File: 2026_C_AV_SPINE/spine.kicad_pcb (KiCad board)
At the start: 4 copper layers, 165 x 80 mm, 165 parts, among them IC1 LT3960EMSE#TRPBF, J1 Conn_01x02_Socket, J10 Conn_01x02_Socket, J11 DIN41612_02x16_AB, J12 SS-12800-009, J13 SS-12800-009, J14 Conn_01x02_Socket, J2 DIN41612_02x16_AB, J3 Conn_01x02_Socket, J4 SS-12800-009, J5 DIN41612_02x16_AB, J6 DIN41612_02x16_AB, J7 Conn_01x02_Socket, J8 SS-12800-009, J9 Conn_01x02_Socket, Q1 PMOS, Q10 SI7972DP-T1-GE3, Q11 SIR5607DP-T1-RE3, Q2 PMOS, Q3 PMOS, Q4 PMOS, Q5 NMOS, Q6 NMOS, Q7 NMOS, Q8 NMOS, Q9 SI7972DP-T1-GE3, U1 INA228, U2 INA228, U3 LTC4418IUF_TRPBF, U4 LM5176RHF, U5 INA228, U6 LTC4020IUHF_PBF

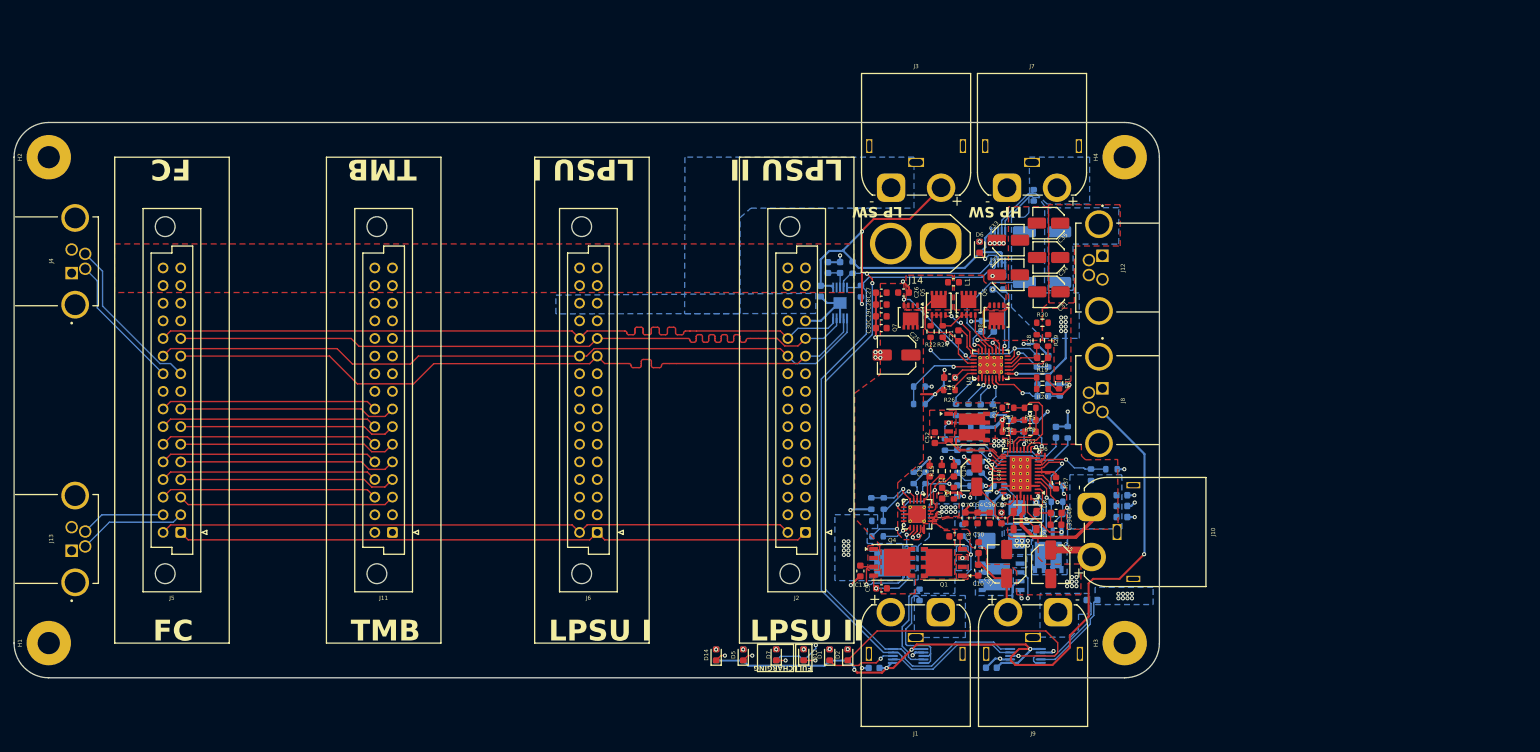
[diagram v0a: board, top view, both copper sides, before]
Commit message: spine almost finished
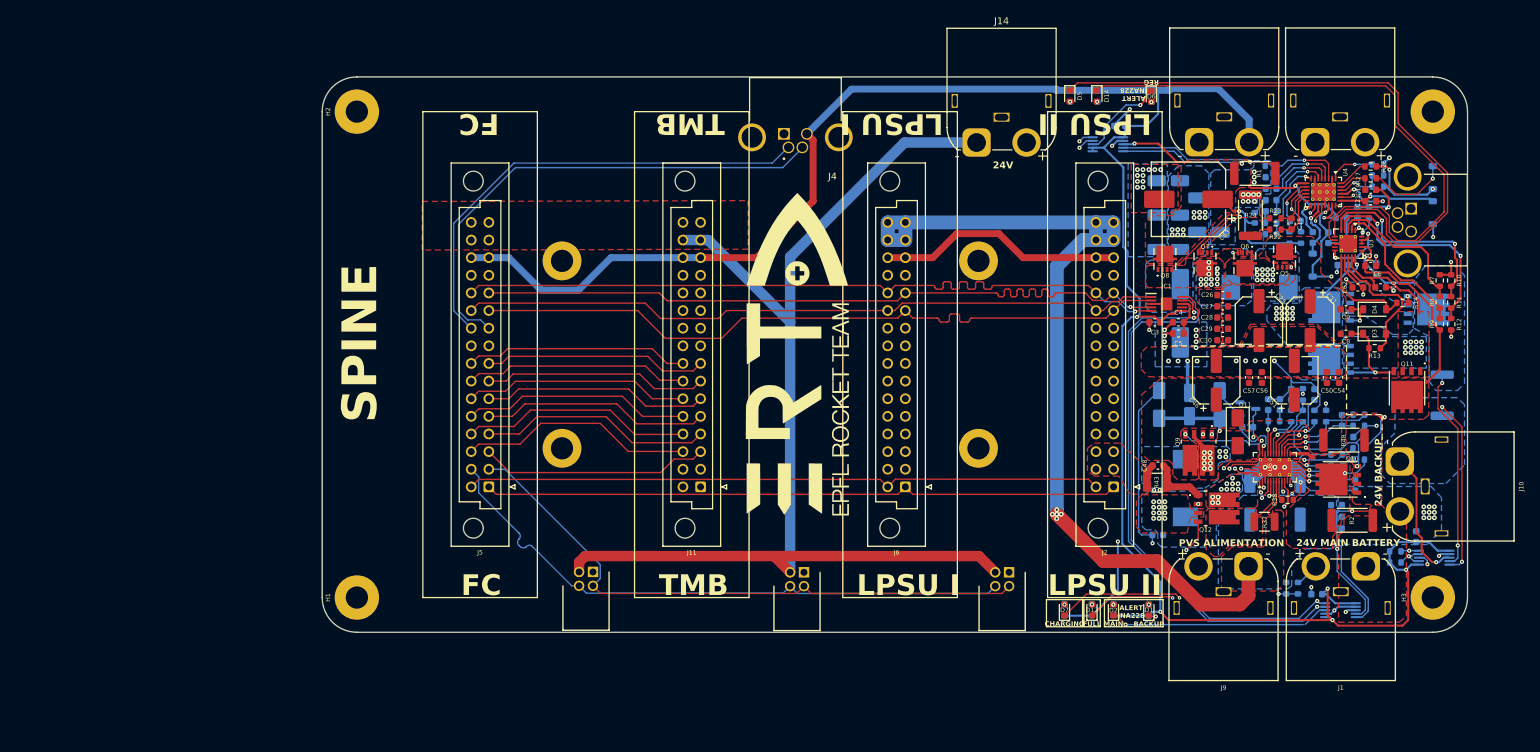
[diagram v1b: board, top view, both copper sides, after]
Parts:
- removed C37: 180u, Capacitor_SMD:C_Elec_6.3x7.7
- removed Q3, Q4: PMOS, Package_SO:PowerPAK_SO-8_Single
- removed R30: 0, Resistor_SMD:R_0603_1608Metric
- added C61: 47u, Capacitor_SMD:CP_Elec_6.3x9.9, B.Cu at (212.8, 119.6)
- added C62: 470n, Capacitor_SMD:C_0603_1608Metric, F.Cu at (221.1, 89.0)
- added C63: 180u, Capacitor_SMD:CP_Elec_10x10.5, F.Cu at (196.7, 76.3)
- added D13: BAT46W-7-F, Diode_SMD:D_SOD-123, B.Cu at (231.9, 78.2)
- added D15: BAT46W-7-F, Diode_SMD:D_SOD-123, B.Cu at (214.6, 85.7)
- added D16: STPS1L60ZF, Diode_SMD:D_SOD-123, B.Cu at (231.9, 73.1)
- added D3: BAT46W-E3-18, Diode_SMD:D_SOD-123, F.Cu at (223.5, 95.6)
- added D4: BAT46W-E3-18, Diode_SMD:D_SOD-123, F.Cu at (223.5, 92.1)
- added G***: LOGO, LOGO, F.Cu at (140.4, 98.6)
- added G***: LOGO, LOGO, B.Cu at (132.2, 123.9)
- added G***: LOGO, LOGO, B.Cu at (109.4, 72.1)
- added G***: LOGO, LOGO, B.Cu at (84.2, 74.4)
- added G***: LOGO, LOGO, B.Cu at (104.7, 121.1)
- added H5: MountingHole_3.2mm_M3_DIN965_Pad, MountingHole:MountingHole_3.2mm_M3_DIN965_Pad, B.Cu at (106.4, 85.1)
- added H6: MountingHole_3.2mm_M3_DIN965_Pad, MountingHole:MountingHole_3.2mm_M3_DIN965_Pad, F.Cu at (166.4, 85.1)
- added H7: MountingHole_3.2mm_M3_DIN965_Pad, MountingHole:MountingHole_3.2mm_M3_DIN965_Pad, F.Cu at (106.4, 112.1)
- added H8: MountingHole_3.2mm_M3_DIN965_Pad, MountingHole:MountingHole_3.2mm_M3_DIN965_Pad, F.Cu at (166.4, 112.1)
- added J15: Conn_02x02, ert:SHDRRA4W55P200_2X2_665X640X630P, F.Cu at (141.3, 130.0)
- added Q12: STL36DN6F7, ert:STL36DN6F7, F.Cu at (200.8, 120.8)
- added Q13: STL42P6LLF6, ert:STL42P6LLF6, B.Cu at (217.1, 99.3)
- C11: value 470n -> 47u; footprint Capacitor_SMD:C_0603_1608Metric -> Capacitor_SMD:CP_Elec_6.3x9.9
- C12: value 220p -> 57p
- C13, C14, C20, C31, C32, C33, C34, C35, C39, C40, C52, C7, R15, R20, R28, R29, R45, R47, R49, R51, R52: moved to B.Cu
- C15, C3, C4, C5, IC1, R12, R13, R14, R23: moved to F.Cu
- C23: value 15n -> 33n
- C24: value 33p -> 560p
- C25: footprint Capacitor_SMD:C_Elec_5x5.8 -> Capacitor_SMD:CP_Elec_6.3x5.9
- C36: footprint Capacitor_SMD:C_Elec_6.3x7.7 -> Capacitor_SMD:CP_Elec_10x10.5
- C44: value 680p -> 10n
- C46: value 1u -> 47u; footprint Capacitor_SMD:C_0603_1608Metric -> Capacitor_SMD:CP_Elec_6.3x9.9
- C48: value 0.033u -> 0.33u; moved to F.Cu
- C51: value 56u -> 47u; footprint Capacitor_SMD:C_Elec_5x5.4 -> Capacitor_SMD:CP_Elec_6.3x9.9
- C55: value 56u -> 47u; footprint Capacitor_SMD:C_Elec_5x5.4 -> Capacitor_SMD:CP_Elec_6.3x9.9; moved to B.Cu
- D10: value MBRS360 -> SZBZX84C6V2LT3G; footprint Diode_SMD:D_SMB -> Package_TO_SOT_SMD:SOT-23-3
- D11: value MBRS360 -> CMSH3-40MA; footprint Diode_SMD:D_SMB -> Diode_SMD:D_SMA; moved to F.Cu
- D8, D9: value SBR0560S1 -> CMSH3-40MA; footprint Diode_SMD:D_SOD-123 -> Diode_SMD:D_SMA; moved to B.Cu
- J12, J13: value SS-12800-009 -> Conn_02x02; footprint ert:STEWART_SS-12800-009 -> ert:SHDRRA4W55P200_2X2_665X640X630P
- J14: footprint Connector_AMASS:AMASS_XT60-F_1x02_P7.20mm_Vertical -> Connector_AMASS:AMASS_XT60IPW-M_1x03_P7.20mm_Horizontal
- J4, J8: value SS-12800-009 -> 54-00274; footprint ert:STEWART_SS-12800-009 -> ert:TENSILITY_54-00274
- L1: value 2u2 -> 1u; footprint Inductor_SMD:L_0603_1608Metric -> Inductor_SMD:L_10.4x10.4_H4.8; moved to B.Cu
- L2: value 15u -> 1u; footprint Inductor_SMD:L_0603_1608Metric -> Inductor_SMD:L_10.4x10.4_H4.8
- Q1: value PMOS -> STL42P6LLF6; footprint Package_SO:PowerPAK_SO-8_Single -> ert:STL42P6LLF6; moved to B.Cu
- Q10: value SI7972DP-T1-GE3 -> STL42P6LLF6; footprint Package_SO:PowerPAK_SO-8_Dual -> ert:STL42P6LLF6; moved to F.Cu
- Q11: value SIR5607DP-T1-RE3 -> STL42P6LLF6; footprint Package_SO:PowerPAK_SO-8_Dual -> ert:STL42P6LLF6
- Q2: value PMOS -> STL42P6LLF6; footprint Package_SO:PowerPAK_SO-8_Single -> ert:STL42P6LLF6
- Q5, Q6, Q7, Q8: value NMOS -> STL8N10F7; footprint Package_TO_SOT_SMD:LFPAK33 -> ert:STL8N10F7
- Q9: value SI7972DP-T1-GE3 -> STL36DN6F7; footprint Package_SO:PowerPAK_SO-8_Dual -> ert:STL36DN6F7; moved to F.Cu
- R1, R2: value 2m -> 10m; footprint Resistor_SMD:R_0603_1608Metric -> Resistor_SMD:R_2512_6332Metric; moved to F.Cu
- R10, R7: value 39k2 -> 40k; moved to F.Cu
- R11, R8: value 10k7 -> 2k5; moved to F.Cu
- R18: value 27k4 -> 15k6
- R19: value 560k -> 597k; moved to B.Cu
- R21: value 20k -> 2k; moved to B.Cu
- R24: value 5m -> 7m; footprint Resistor_SMD:R_0603_1608Metric -> Resistor_SMD:R_2512_6332Metric
- R27: value 2k -> 10; moved to F.Cu
- R31: value 59k -> 10k
- R34: value 2m -> 10m; footprint Resistor_SMD:R_0603_1608Metric -> Resistor_SMD:R_2512_6332Metric
- R37: value 5m -> 3m; footprint Resistor_SMD:R_0603_1608Metric -> Resistor_SMD:R_1210_3225Metric
- R38: value 100k -> 50k; moved to F.Cu
- R43: value 5m -> 3m; footprint Resistor_SMD:R_0603_1608Metric -> Resistor_SMD:R_1210_3225Metric; moved to F.Cu
- R48: value 10m -> 12m; footprint Resistor_SMD:R_0603_1608Metric -> Resistor_SMD:R_2512_6332Metric; moved to F.Cu
- R53: value 82k5 -> 80k; moved to B.Cu
- R54: value 20k -> 47k5
- U6: footprint Package_DFN_QFN:WQFN-38-1EP_5x7mm_P0.5mm_EP3.15x5.15mm_ThermalVias -> Package_DFN_QFN:QFN-38-1EP_4x6mm_P0.4mm_EP2.65x4.65mm_ThermalVias
- moved J4 105.3 mm to (140.1, 67.3), turned to 180 degrees
- moved R17 97.4 mm to (183.5, 61.4), turned to 90 degrees
- moved D14 97.4 mm to (183.5, 61.4), turned to -90 degrees
- moved R16 93.3 mm to (179.6, 61.4), turned to 90 degrees
- moved D5 93.2 mm to (179.6, 61.4), turned to -90 degrees
- moved R10 89.5 mm to (234.5, 88.0), turned to 90 degrees
- moved R5 88.2 mm to (226.5, 127.0), turned to 0 degrees
- moved R12 87.4 mm to (234.5, 94.3), turned to 90 degrees
- moved R11 86.7 mm to (234.5, 91.1)
- moved R6 86.3 mm to (226.5, 128.6), turned to 0 degrees
- moved R14 82.8 mm to (227.5, 91.2), turned to 180 degrees
- moved R7 80.9 mm to (232.9, 88.0)
- moved R34 80.6 mm to (233.2, 104.5)
- moved C38 80.4 mm to (229.5, 124.9), turned to -90 degrees
- moved Q1 78.6 mm to (231.1, 92.1), turned to 90 degrees
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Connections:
- net /Power/Charger/D_1 renamed /Power/Charger/SENSTOP
- net /Power/Charger/VBG renamed /Power/Charger/FBG
- net Net-(U6-ITH) renamed /Power/Charger/ITH
- net Net-(U6-RNG/SS) renamed /Power/Charger/RNG/SS
- net Net-(U6-TIMER) renamed /Power/Charger/TIMER
- net Net-(U6-VC) renamed /Power/Charger/VC
- C11 pad 1: GND -> /Power/Management/24V_MUXOUT
- C11 pad 2: /Power/Management/VS2 -> GND
- C18 pad 1: /Power/Management/24V_OUT_REG -> 24V_OUT_REG
- C31 pad 1: GND -> 24V_OUT_REG
- C31 pad 2: /Power/Management/QH2OUT -> GND
- C32 pad 1: GND -> 24V_OUT_REG
- C32 pad 2: /Power/Management/QH2OUT -> GND
- C33 pad 1: GND -> 24V_OUT_REG
- C33 pad 2: /Power/Management/QH2OUT -> GND
- C34 pad 1: GND -> 24V_OUT_REG
- C34 pad 2: /Power/Management/QH2OUT -> GND
- C35 pad 1: GND -> 24V_OUT_REG
- C35 pad 2: /Power/Management/QH2OUT -> GND
- C36 pad 1: GND -> 24V_OUT_REG
- C36 pad 2: /Power/Management/24V_OUT_REG -> GND
- C39 pad 2: /Power/Charger/D_2 -> /Power/Charger/SW1
- C41 pad 1: /Power/Charger/D_4 -> /Power/Charger/SW2
- C46 pad 1: /Power/Charger/D_2 -> VOUT_CHARG
- C46 pad 2: /Power/Charger/BST1 -> GND
- C48 pad 1: /Power/Charger/S_2 -> /Power/Charger/SENSBOT
- C50 pad 1: /Power/Charger/24V_OUT_CHARG -> VOUT_CHARG
- C51 pad 1: GND -> VOUT_CHARG
- C51 pad 2: /Power/Charger/24V_OUT_CHARG -> GND
- C52 pad 1: /Power/Charger/G_5 -> /Power/Charger/BGATE
- C54 pad 1: /Power/Charger/24V_OUT_CHARG -> VOUT_CHARG
- C55 pad 1: GND -> 24V_PFS
- C55 pad 2: /Power/Charger/24V_OUT_CHARG -> GND
- C56 pad 1: /Power/Charger/24V_OUT_CHARG -> VOUT_CHARG
- C57 pad 1: /Power/Charger/24V_OUT_CHARG -> VOUT_CHARG
- C6 pad 2: 24V_BATT_BCK -> VOUT_CHARG
- C7 pad 1: /Power/Charger/24V_OUT_CHARG -> 24V_BATT_BCK
- C8 pad 2: /Power/Management/G1 -> /Power/Management/G1MOS
- C9 pad 2: /Power/Management/G2 -> /Power/Management/G2MOS
- D10 pad 2: /Power/Charger/D_4 -> /Power/Charger/SW2
- D11 pad 1: /Power/Charger/24V_OUT_CHARG -> VOUT_CHARG
- D11 pad 2: /Power/Charger/D_4 -> /Power/Charger/SW2
- D8 pad 1: /Power/Charger/BST1 -> /Power/Charger/BST2
- D9 pad 1: /Power/Charger/BST2 -> /Power/Charger/BST1
- J1 pad 1: 24V_BATT_BCK_IN -> 24V_BATT_IN
- J10 pad 1: 24V_PFS -> 24V_BATT_BCK_IN
- J12 pad 2: /Connectors/INTRANET_CAN_H -> /Connectors/CAM_CAN_H
- J12 pad 3: /Connectors/INTRANET_CAN_L -> +24V
- J12 pad 4: +5V -> /Connectors/CAM_CAN_L
- J13 pad 3: /Connectors/CAM_CAN_L -> +24V
- J13 pad 4: +5V -> /Connectors/CAM_CAN_L
- J2 pad a15: +24V -> 24V_PFS
- J2 pad a16: +24V -> 24V_PFS
- J2 pad b15: +24V -> 24V_PFS
- J2 pad b16: +24V -> 24V_PFS
- J4 pad 3: /Connectors/RS232_FDR_TX -> +5V
- J4 pad 4: +5V -> /Connectors/RS232_FDR_TX
- J6 pad a15: +24V -> 24V_PFS
- J6 pad a16: +24V -> 24V_PFS
- J6 pad b15: +24V -> 24V_PFS
- J6 pad b16: +24V -> 24V_PFS
- J8 pad 3: /Connectors/INTRANET_CAN_L -> +5V
- J8 pad 4: +5V -> /Connectors/INTRANET_CAN_L
- J9 pad 1: 24V_BATT_IN -> 24V_PFS
- L2 pad 1: /Power/Charger/D_2 -> /Power/Charger/SW1
- L2 pad 2: /Power/Charger/D_4 -> /Power/Charger/SW2
- Q1 pad 1: /Power/Management/24V_MUXOUT -> /Power/Management/VS2
- Q1 pad 2: /Power/Management/G1 -> /Power/Management/VS2
- Q1 pad 3: /Power/Management/VS1 -> /Power/Management/VS2
- Q10 pad 1: /Power/Charger/D_4 -> /Power/Charger/S_5
- Q10 pad 2: /Power/Charger/G_3 -> /Power/Charger/S_5
- Q10 pad 3: GND -> /Power/Charger/S_5
- Q10 pad 4: /Power/Charger/G_4 -> /Power/Charger/BGATE
- Q10 pad 5: /Power/Charger/D_4 -> 24V_BATT
- Q10 pad 6: /Power/Charger/D_4 -> 24V_BATT
- Q11 pad 1: /Power/Charger/S_5 -> /Power/Management/VS1
- Q11 pad 2: /Power/Charger/S_5 -> /Power/Management/VS1
- Q11 pad 3: /Power/Charger/S_5 -> /Power/Management/VS1
- Q11 pad 4: /Power/Charger/G_5 -> /Power/Management/G1MOS
- Q11 pad 5: 24V_BATT -> VOUT_CHARG
- Q11 pad 6: 24V_BATT -> VOUT_CHARG
- Q2 pad 1: 24V_BATT_BCK -> /Power/Management/VS2
- Q2 pad 2: /Power/Management/G1 -> /Power/Management/VS2
- Q2 pad 3: /Power/Management/VS1 -> /Power/Management/VS2
- Q5 pad 2: /Power/Management/LDRV1 -> /Power/Management/SW1
- Q5 pad 3: /Power/Management/RSENSE -> /Power/Management/SW1
- Q6 pad 1: /Power/Management/SW2 -> /Power/Management/RSENSE
- Q6 pad 2: /Power/Management/LDRV2 -> /Power/Management/RSENSE
- Q7 pad 1: /Power/Management/24V_MUXOUT -> /Power/Management/RSENSE
- Q7 pad 2: /Power/Management/HDRV1 -> /Power/Management/RSENSE
- Q7 pad 3: /Power/Management/SW1 -> /Power/Management/RSENSE
- Q8 pad 1: /Power/Management/QH2OUT -> /Power/Management/SW2
- Q8 pad 2: /Power/Management/HDRV2 -> /Power/Management/SW2
- Q9 pad 1: /Power/Charger/D_2 -> GND
- Q9 pad 2: /Power/Charger/G_1 -> /Power/Charger/BG2
- Q9 pad 3: /Power/Charger/S_2 -> /Power/Charger/SW2
- Q9 pad 4: /Power/Charger/G_2 -> /Power/Charger/TG2
- Q9 pad 5: /Power/Charger/D_2 -> VOUT_CHARG
- Q9 pad 6: /Power/Charger/D_2 -> VOUT_CHARG
- R1 pad 1: /Power/Management/24V_OUT_REG -> 24V_OUT_REG
- R12 pad 1: /Power/Charger/24V_OUT_CHARG -> 24V_BATT_BCK
- R13 pad 1: /Power/Management/G1 -> /Power/Management/G1MOS
- R13 pad 2: Net-(D3-A) -> /Power/Management/G1
- R14 pad 1: /Power/Management/G2 -> /Power/Management/G2MOS
- R14 pad 2: Net-(D4-A) -> /Power/Management/G2
- R21 pad 2: /Power/Management/24V_OUT_REG -> 24V_OUT_REG
- R27 pad 1: /Power/Management/24V_MUXOUT -> Net-(D16-K)
- R28 pad 1: /Power/Management/QH2OUT -> 24V_OUT_REG
- R29 pad 2: /Power/Management/24V_OUT_REG -> 24V_OUT_REG
- R38 pad 1: Net-(U6-RT) -> GND
- R38 pad 2: GND -> /Power/Charger/RT
- R43 pad 1: /Power/Charger/S_2 -> /Power/Charger/SENSBOT
- R44 pad 1: /Power/Charger/24V_OUT_CHARG -> VOUT_CHARG
- R48 pad 1: /Power/Charger/24V_OUT_CHARG -> VOUT_CHARG
- R51 pad 2: /Power/Charger/24V_OUT_CHARG -> VOUT_CHARG
- R53 pad 2: /Power/Charger/24V_OUT_CHARG -> VOUT_CHARG
- R9 pad 1: 24V_BATT_BCK -> VOUT_CHARG
- U1 pad 10: /Power/Management/24V_OUT_REG -> 24V_OUT_REG
- U1 pad 8: /Power/Management/24V_OUT_REG -> 24V_OUT_REG
- U3 pad 11: Net-(D4-A) -> /Power/Management/G2
- U3 pad 13: Net-(D3-A) -> /Power/Management/G1
- U3 pad 16: /Power/Charger/24V_OUT_CHARG -> 24V_BATT_BCK
- U3 pad 17: 24V_BATT_BCK -> VOUT_CHARG
- U4 pad 21: /Power/Management/24V_OUT_REG -> 24V_OUT_REG
- U4 pad 9: /Power/Management/24V_OUT_REG -> 24V_OUT_REG
- U6 pad 1: /Power/Charger/G_1 -> /Power/Charger/TG1
- U6 pad 21: /Power/Charger/G_5 -> /Power/Charger/BGATE
- U6 pad 31: /Power/Charger/G_3 -> /Power/Charger/TG2
- U6 pad 32: /Power/Charger/D_4 -> /Power/Charger/SW2
- U6 pad 33: /Power/Charger/G_4 -> /Power/Charger/BG2
- U6 pad 37: /Power/Charger/G_2 -> /Power/Charger/BG1
- U6 pad 38: /Power/Charger/D_2 -> /Power/Charger/SW1
- U6 pad 5: /Power/Charger/S_2 -> /Power/Charger/SENSBOT
- U6 pad 8: Net-(U6-RT) -> /Power/Charger/RT
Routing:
- net +5V: track 189.2 -> 361.0 mm, vias 7 -> 5
- net +24V: track 0.00 -> 165.4 mm
- net 24V_PFS: track 23.1 -> 151.2 mm, vias 0 -> 7
- net /Connectors/CAM_CAN_L: track 12.2 -> 86.9 mm
- net /Connectors/CAM_CAN_H: track 15.7 -> 86.9 mm
- net 24V_OUT_REG: track 0.00 -> 70.4 mm, vias 0 -> 17
- net /Connectors/5Vin: track 0.32 -> 60.3 mm
- net /Power/Management/VALID1: track 34.5 -> 93.1 mm, vias 2 -> 0
- net /Power/Management/VALID2: track 37.6 -> 89.4 mm, vias 2 -> 0
- net /Connectors/RS232_FDR_RX: track 19.8 -> 68.8 mm
- net /Connectors/RS232_FDR_TX: track 23.9 -> 72.0 mm
- net /Power/Management/24V_OUT_REG: track 42.9 -> 0.00 mm, vias 10 -> 0
- net /Power/Charger/BST1: track 7.96 -> 49.3 mm, vias 0 -> 2
- net /Power/Management/VCC: track 5.13 -> 44.5 mm, vias 1 -> 3
- net VOUT_CHARG: track 0.00 -> 36.2 mm, vias 0 -> 3
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- added copper zone on F.Cu, net /Power/Charger/SENSTOP
- added copper zone on B.Cu, net /Power/Charger/SW1
- added copper zone on F.Cu, net /Power/Charger/SW1
- added copper zone on B.Cu, net /Power/Charger/SW2
- added copper zone on F.Cu, net /Power/Charger/SW2
- added copper zone on B.Cu, net /Power/Management/24V_MUXOUT
- added copper zone on F.Cu, net /Power/Management/RSENSE
- added copper zone on B.Cu, net /Power/Management/SW1
- added copper zone on B.Cu, net /Power/Management/SW2
- added copper zone on F.Cu, net 24V_BATT_IN
- added copper zone on B.Cu, net 24V_OUT_REG
- added copper zone on F.Cu, net 24V_OUT_REG
- added copper zone on F.Cu, net VOUT_CHARG
- removed copper zone on In1.Cu, net +24V
- removed copper zone on B.Cu, net +24V_SW
- removed copper zone on In1.Cu, net +5V
- removed copper zone on B.Cu, net /Connectors/5Vin
- removed copper zone on B.Cu, net /Power/Charger/24V_OUT_CHARG
- removed copper zone on F.Cu, net /Power/Charger/24V_OUT_CHARG
- removed copper zone on In1.Cu, net /Power/Charger/24V_OUT_CHARG
- removed copper zone on B.Cu, net /Power/Charger/D_2
- removed copper zone on B.Cu, net /Power/Charger/D_4
- removed copper zone on B.Cu, net /Power/Management/24V_OUT_REG
- removed copper zone on F.Cu, net /Power/Management/24V_OUT_REG
- removed copper zone on F.Cu, net /Power/Management/QH2OUT
- removed copper zone on F.Cu, net /Power/Management/VS2
- removed copper zone on B.Cu, net 24V_BATT
- removed copper zone on In2.Cu, net 24V_BATT
- removed copper zone on F.Cu, net 24V_BATT_BCK
- removed copper zone on B.Cu, net 24V_BATT_IN
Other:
- board text added: "24V"
- board text added: "24V BACKUP"
- board text added: "24V MAIN BATTERY"
- board text added: "ALERT INA228"
- board text added: "BACKUP"
- board text added: "CATS"
- board text added: "MAIN"
- board text added: "PVS ALIMENTATION"
- board text added: "REG"
- board text added: "SPINE"
- board text removed: "HP SW"
- board text removed: "LP SW"
